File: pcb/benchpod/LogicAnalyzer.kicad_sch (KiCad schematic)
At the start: 54 parts, among them U18 SN74LVC2G66DCUR, U19 SN74LVC2G66DCUR, U20 SN74LVC2G66DCUR, U21 SN74LVC2G66DCUR, U22 SRV05-4.TCT, U23 SRV05-4.TCT, U25 SRV05-4.TCT, U34 SRV05-4.TCT, U54 TCA9554PWR

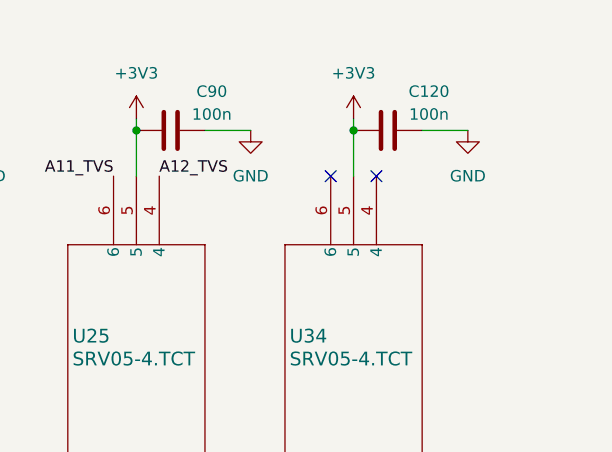
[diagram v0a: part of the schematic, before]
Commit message: esd fixes
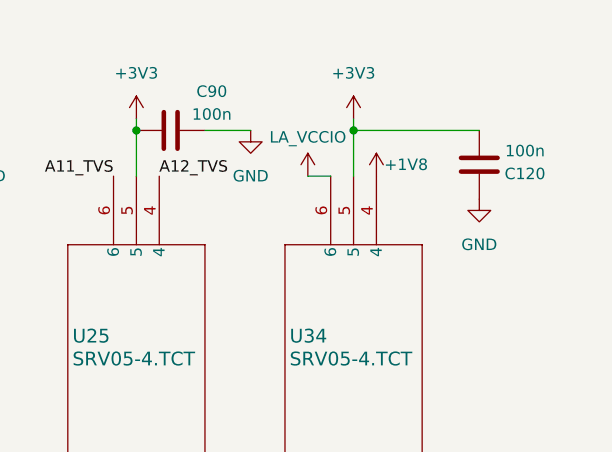
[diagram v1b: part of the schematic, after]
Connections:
- net +3V3: now also C120.2; no longer C120.1
- net GND: now also C120.1; no longer C120.2
- net LA_VCCIO: now also U34.6
- net +1V8: now reaches U34.4
- no-connect marks 2 -> 0
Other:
- moved on the sheet: C120
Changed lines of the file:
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@@
 	)
 	(junction
-		(at 256.54 33.02)
-		(diameter 0)
-		(color 0 0 0 0)
-	)
-	(junction
 		(at 78.74 157.48)
 		(diameter 0)
@@
 	)
 	(junction
+		(at 256.54 33.02)
+		(diameter 0)
+		(color 0 0 0 0)
+	)
+	(junction
 		(at 110.49 130.81)
 		(diameter 0)
@@
 		(color 0 0 0 0)
 	)
-	(no_connect
-		(at 254 38.1)
-	)
-	(no_connect
-		(at 259.08 38.1)
-	)
 	(wire
 		(pts
@@
 	(wire
 		(pts
+			(xy 251.46 38.1) (xy 254 38.1)
+		)
+		(stroke
+			(width 0)
+			(type default)
+		)
+	)
+	(wire
+		(pts
 			(xy 66.04 129.54) (xy 66.04 135.89)
 		)
@@
 	(wire
 		(pts
-			(xy 269.24 33.02) (xy 264.16 33.02)
-		)
-		(stroke
-			(width 0)
-			(type default)
-		)
-	)
-	(wire
-		(pts
 			(xy 139.7 125.73) (xy 138.43 125.73)
 		)
@@
 	(wire
 		(pts
+			(xy 256.54 33.02) (xy 270.51 33.02)
+		)
+		(stroke
+			(width 0)
+			(type default)
+		)
+	)
+	(wire
+		(pts
 			(xy 60.96 157.48) (xy 60.96 170.18)
 		)
@@
 	)
 	(symbol
+		(lib_id "power:+3V3")
+		(at 251.46 38.1 0)
+		(unit 1)
+		(body_style 1)
+		(exclude_from_sim no)
+		(in_bom yes)
+		(on_board yes)
+		(in_pos_files yes)
+		(dnp no)
+		(property "Reference" "#PWR0351"
+			(at 251.46 41.91 0)
+			(hide yes)
+			(show_name no)
+			(do_not_autoplace no)
+			(effects
+				(font
+					(size 1.27 1.27)
+				)
+			)
+		)
+		(property "Value" "LA_VCCIO"
+			(at 251.46 33.782 0)
+			(show_name no)
+			(do_not_autoplace no)
+			(effects
+				(font
+					(size 1.27 1.27)
+				)
+			)
+		)
+		(property "Footprint" ""
+			(at 251.46 38.1 0)
+			(hide yes)
+			(show_name no)
+			(do_not_autoplace no)
+			(effects
+				(font
+					(size 1.27 1.27)
+				)
+			)
+		)
+		(property "Datasheet" ""
+			(at 251.46 38.1 0)
+			(hide yes)
+			(show_name no)
+			(do_not_autoplace no)
+			(effects
+				(font
+					(size 1.27 1.27)
+				)
+			)
+		)
+		(property "Description" "Power symbol creates a global label with name \"+3V3\""
+			(at 251.46 38.1 0)
+			(hide yes)
+			(show_name no)
+			(do_not_autoplace no)
+			(effects
+				(font
+					(size 1.27 1.27)
+				)
+			)
+		)
+		(pin "1"
+		)
+		(instances
+			(project "vbench-pod"
+				(path "/745fcf4b-2e0b-4fc4-95c0-f2e3fd40beb9/e3454fef-24e2-422b-9513-46b286a60c18"
+					(reference "#PWR0351")
+					(unit 1)
+				)
+			)
+		)
+	)
+	(symbol
 		(lib_id "Device:R")
 		(at 162.56 132.08 0)
@@
 	(symbol
 		(lib_id "power:GND")
-		(at 269.24 33.02 0)
+		(at 270.51 40.64 0)
 		(unit 1)
 		(body_style 1)
@@
 		(fields_autoplaced yes)
 		(property "Reference" "#PWR0202"
-			(at 269.24 39.37 0)
+			(at 270.51 46.99 0)
 			(hide yes)
 			(show_name no)
@@
 		)
 		(property "Value" "GND"
-			(at 269.24 38.1 0)
+			(at 270.51 45.72 0)
 			(show_name no)
 			(do_not_autoplace no)
@@
 		)
 		(property "Footprint" ""
-			(at 269.24 33.02 0)
+			(at 270.51 40.64 0)
 			(hide yes)
 			(show_name no)
@@
 		)
 		(property "Datasheet" ""
-			(at 269.24 33.02 0)
+			(at 270.51 40.64 0)
 			(hide yes)
 			(show_name no)
@@
 		)
 		(property "Description" "Power symbol creates a global label with name \"GND\" , ground"
-			(at 269.24 33.02 0)
+			(at 270.51 40.64 0)
 			(hide yes)
 			(show_name no)
@@
 	(symbol
 		(lib_id "Device:C")
-		(at 260.35 33.02 90)
+		(at 270.51 36.83 180)
 		(unit 1)
 		(body_style 1)
@@
 		(dnp no)
 		(property "Reference" "C120"
-			(at 264.922 28.702 90)
+			(at 275.59 37.846 0)
 			(show_name no)
 			(do_not_autoplace no)
@@
 		)
 		(property "Value" "100n"
-			(at 264.922 31.242 90)
+			(at 275.59 35.306 0)
 			(show_name no)
 			(do_not_autoplace no)
@@
 		)
 		(property "Footprint" "Capacitor_SMD:C_0402_1005Metric"
-			(at 264.16 32.0548 0)
+			(at 269.5448 33.02 0)
 			(hide yes)
 			(show_name no)
@@
 		)
 		(property "Datasheet" ""
-			(at 260.35 33.02 0)
+			(at 270.51 36.83 0)
 			(hide yes)
 			(show_name no)
@@
 		)
 		(property "Description" "Unpolarized capacitor"
-			(at 260.35 33.02 0)
+			(at 270.51 36.83 0)
 			(hide yes)
 			(show_name no)
@@
 		)
 		(property "LCSC" "C307331"
-			(at 260.35 33.02 90)
+			(at 270.51 36.83 90)
 			(hide yes)
 			(show_name no)
@@
 		)
 		(property "LCSC Part #" ""
-			(at 260.35 33.02 90)
+			(at 270.51 36.83 90)
 			(hide yes)
 			(show_name no)
@@
 		)
 		(property "MFR. Part #" ""
-			(at 260.35 33.02 90)
+			(at 270.51 36.83 90)
 			(hide yes)
 			(show_name no)
@@
 		)
 		(property "KiLib_Generator" "SMD_2terminal_chip_molded"
-			(at 260.35 33.02 0)
+			(at 270.51 36.83 0)
 			(hide yes)
 			(show_name no)
@@
 		)
 		(property "Arrow Part Number" ""
-			(at 260.35 33.02 90)
+			(at 270.51 36.83 90)
 			(hide yes)
 			(show_name no)
@@
 		)
 		(property "Arrow Price/Stock" ""
-			(at 260.35 33.02 90)
+			(at 270.51 36.83 90)
 			(hide yes)
 			(show_name no)
@@
 		)
 		(property "Height" ""
-			(at 260.35 33.02 90)
+			(at 270.51 36.83 90)
 			(hide yes)
 			(show_name no)
@@
 		)
 		(property "Manufacturer_Name" ""
-			(at 260.35 33.02 90)
+			(at 270.51 36.83 90)
 			(hide yes)
 			(show_name no)
@@
 		)
 		(property "Manufacturer_Part_Number" ""
-			(at 260.35 33.02 90)
+			(at 270.51 36.83 90)
 			(hide yes)
 			(show_name no)
@@
 		)
 		(property "Mouser Part Number" ""
-			(at 260.35 33.02 90)
+			(at 270.51 36.83 90)
 			(hide yes)
 			(show_name no)
@@
 		)
 		(property "Mouser Price/Stock" ""
-			(at 260.35 33.02 90)
+			(at 270.51 36.83 90)
 			(hide yes)
 			(show_name no)
@@
 		)
 		(property "ProductID" ""
-			(at 260.35 33.02 90)
+			(at 270.51 36.83 90)
 			(hide yes)
 			(show_name no)
@@
 		)
 		(property "Sim.Pins" ""
-			(at 260.35 33.02 90)
+			(at 270.51 36.83 90)
 			(hide yes)
 			(show_name no)
@@
 		)
 		(property "KLC_S3.3" ""
-			(at 260.35 33.02 90)
+			(at 270.51 36.83 90)
 			(hide yes)
 			(show_name no)
@@
 		)
 		(property "KLC_S4.1" ""
-			(at 260.35 33.02 90)
+			(at 270.51 36.83 90)
 			(hide yes)
 			(show_name no)
@@
 					(unit 1)
 				)
+			)
+		)
+	)
+	(symbol
+		(lib_id "power:+3V3")
+		(at 259.08 38.1 0)
+		(unit 1)
+		(body_style 1)
+		(exclude_from_sim no)
+		(in_bom yes)
+		(on_board yes)
+		(in_pos_files yes)
+		(dnp no)
+		(property "Reference" "#PWR0366"
+			(at 259.08 41.91 0)
+			(hide yes)
+			(show_name no)
+			(do_not_autoplace no)
+			(effects
+				(font
+					(size 1.27 1.27)
+				)
+			)
+		)
+		(property "Value" "+1V8"
+			(at 262.382 36.83 0)
+			(show_name no)
+			(do_not_autoplace no)
+			(effects
+				(font
+					(size 1.27 1.27)
+				)
+			)
+		)
+		(property "Footprint" ""
+			(at 259.08 38.1 0)
+			(hide yes)
+			(show_name no)
+			(do_not_autoplace no)
+			(effects
+				(font
+					(size 1.27 1.27)
+				)
+			)
+		)
+		(property "Datasheet" ""
+			(at 259.08 38.1 0)
+			(hide yes)
+			(show_name no)
+			(do_not_autoplace no)
+			(effects
+				(font
+					(size 1.27 1.27)
+				)
+			)
+		)
+		(property "Description" "Power symbol creates a global label with name \"+3V3\""
+			(at 259.08 38.1 0)
+			(hide yes)
+			(show_name no)
+			(do_not_autoplace no)
+			(effects
+				(font
+					(size 1.27 1.27)
+				)
+			)
+		)
+		(pin "1"
+		)
+		(instances
+			(project "vbench-pod"
+				(path "/745fcf4b-2e0b-4fc4-95c0-f2e3fd40beb9/e3454fef-24e2-422b-9513-46b286a60c18"
+					(reference "#PWR0366")
+					(unit 1)
+				)
